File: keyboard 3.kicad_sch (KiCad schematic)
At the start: 9 parts, among them SW1 SW_Push, SW2 SW_Push, SW3 SW_Push, SW4 SW_Push, SW5 SW_Push, SW6 SW_Push, U1 XIAO-RP2040-DIP

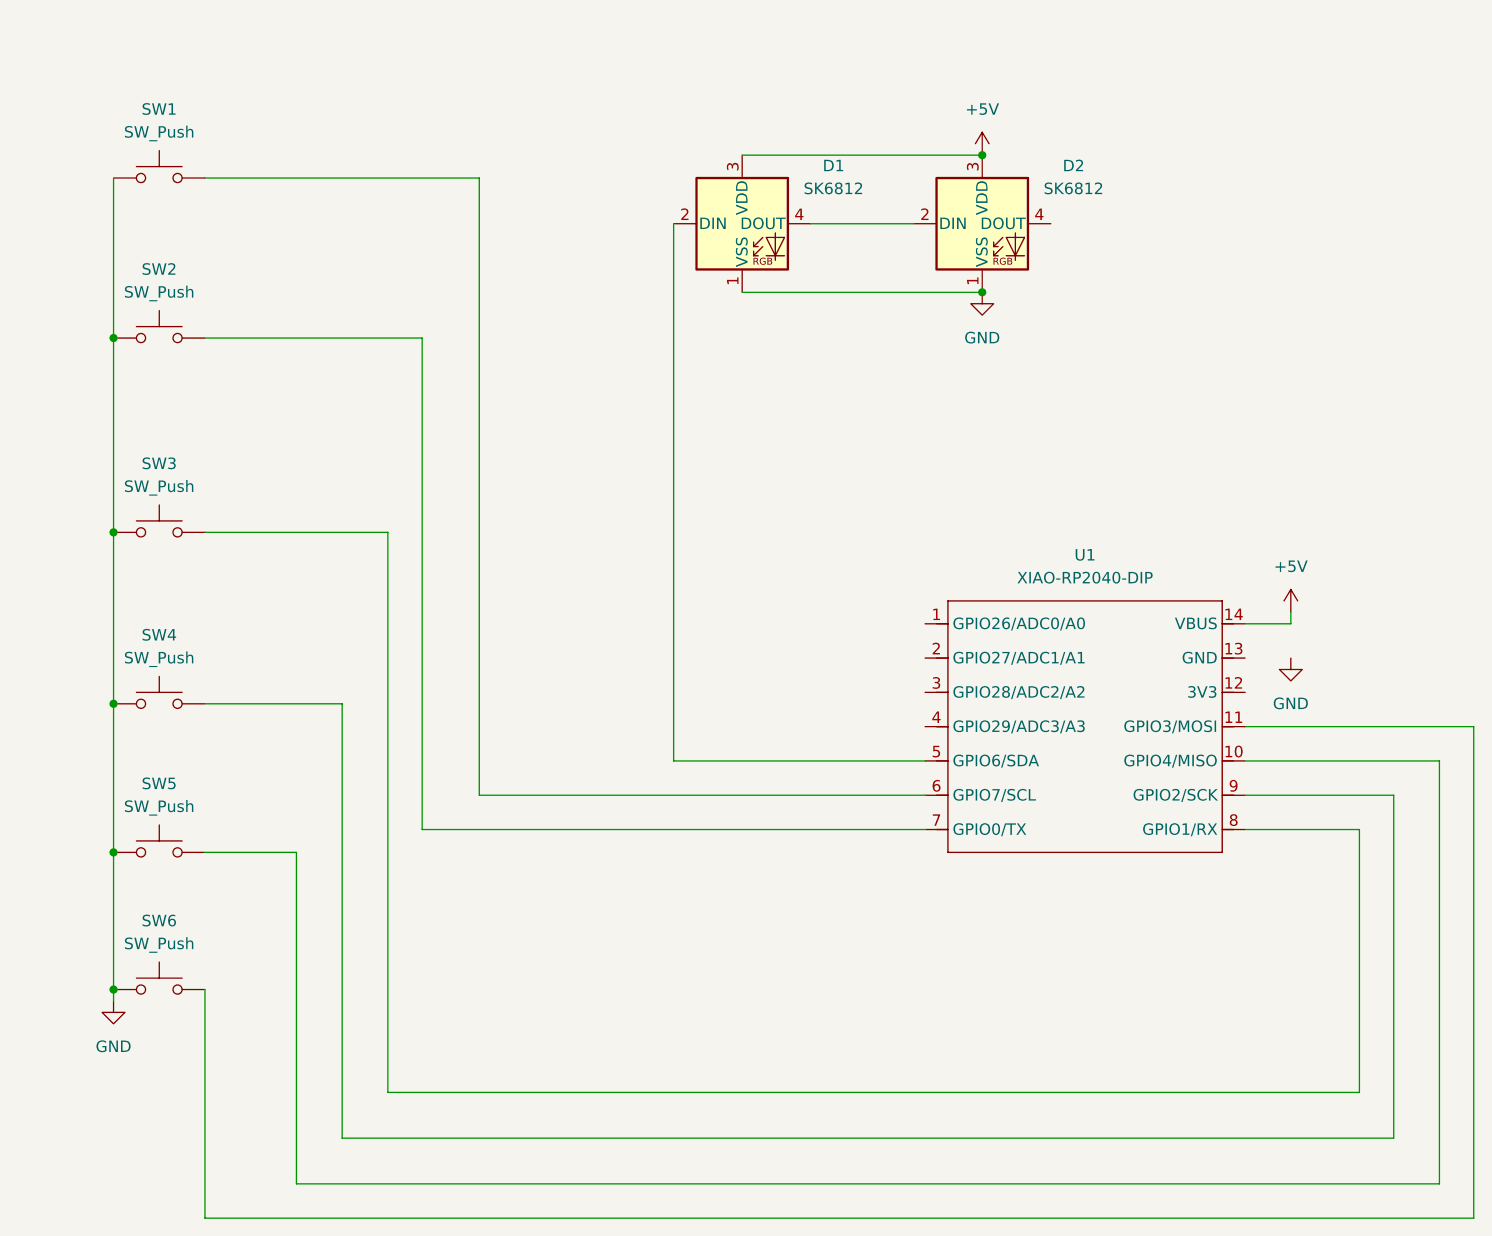
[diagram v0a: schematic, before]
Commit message: Add files via upload
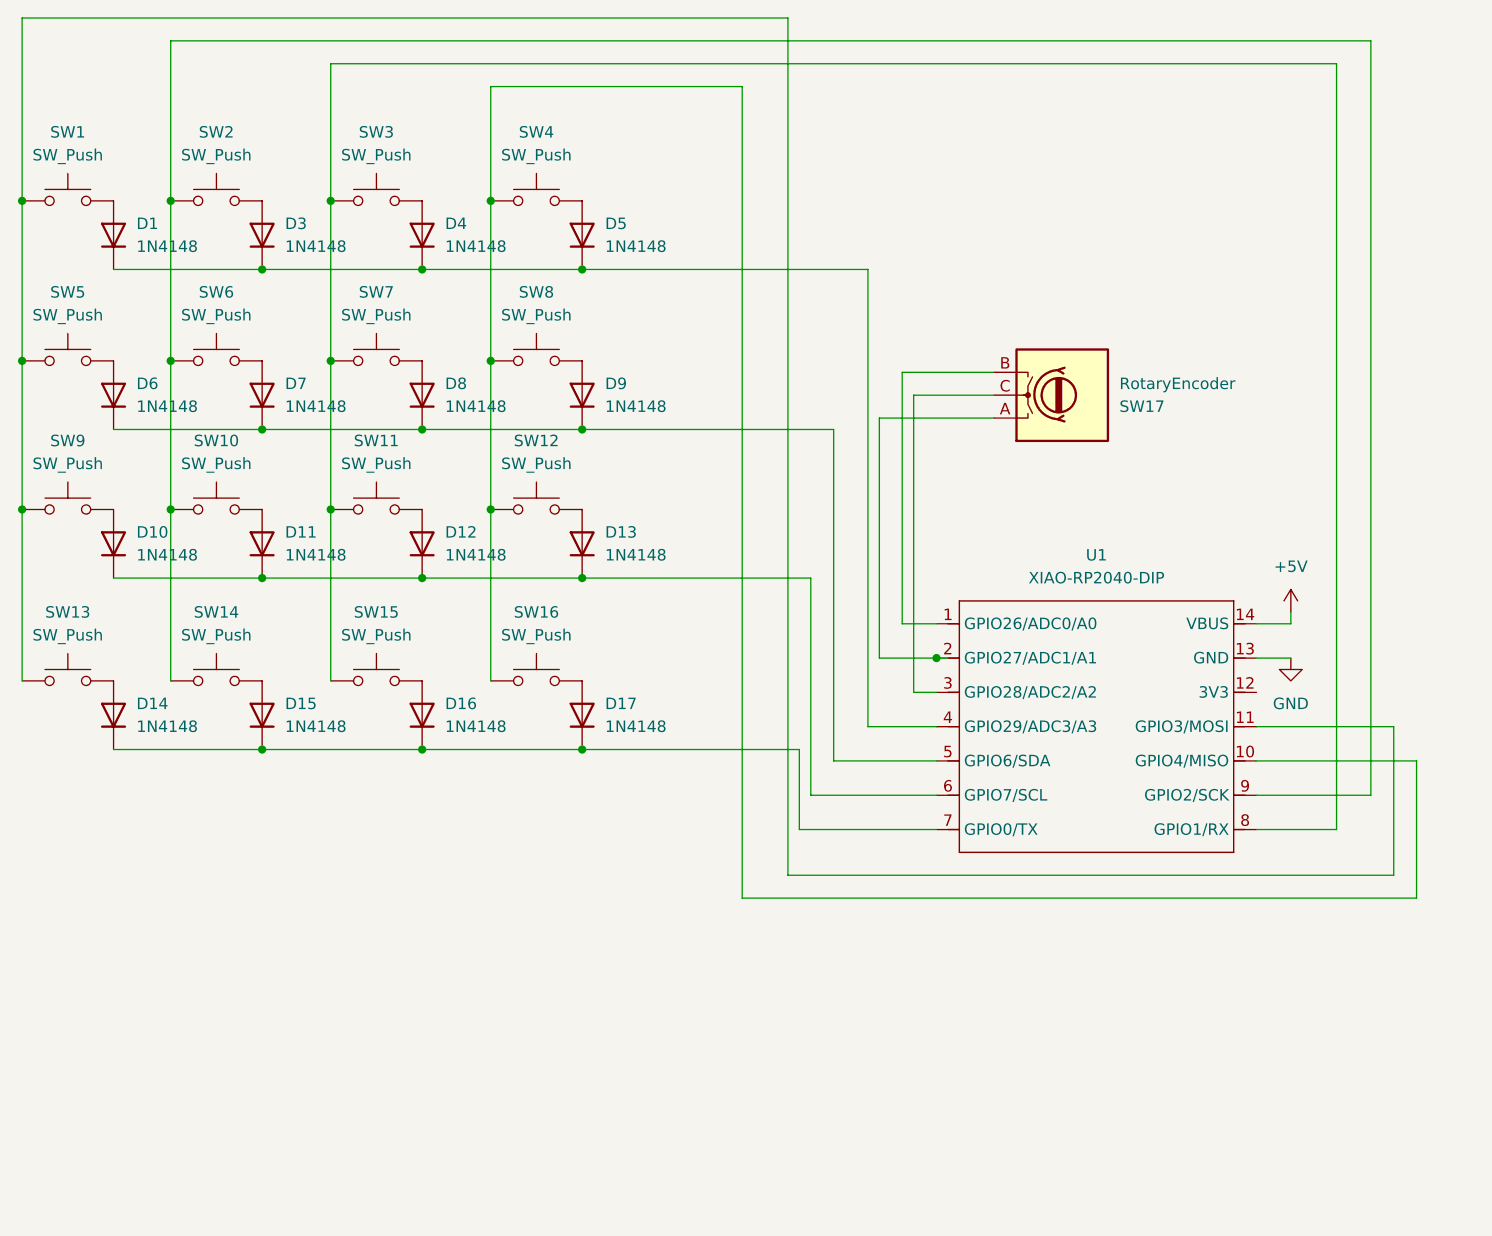
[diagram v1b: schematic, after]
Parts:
- removed D1, D2: SK6812, LED_SMD:LED_SK6812MINI_PLCC4_3.5x3.5mm_P1.75mm, symbol LED:SK6812
- added D1, D10, D11, D12, D13, D14, D15, D16, D17, D3, D4, D5, D6, D7, D8, D9: 1N4148, Diode_THT:D_DO-35_SOD27_P7.62mm_Horizontal, symbol Diode:1N4148
- added SW10, SW11, SW12, SW13, SW14, SW15, SW16, SW7, SW8, SW9: SW_Push, Button_Switch_Keyboard:SW_Cherry_MX_1.00u_PCB, symbol Switch:SW_Push
- added SW17: RotaryEncoder, Rotary_Encoder:RotaryEncoder_Alps_EC11E-Switch_Vertical_H20mm, symbol Device:RotaryEncoder
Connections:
- net GND: now also U1.13 (GND); no longer SW1.1, SW2.1, SW3.1, SW4.1, SW5.1, SW6.1
- net at U1.6 (GPIO7/SCL): now also D10.1 (K), D11.1 (K), D12.1 (K), D13.1 (K); no longer SW1.2
- net at U1.11 (GPIO3/MOSI): now also SW1.1, SW5.1, SW13.1, SW9.1; no longer SW6.2
- net at SW2.2: now also D3.2 (A); no longer U1.7 (GPIO0/TX)
- net at SW3.2: now also D4.2 (A); no longer U1.8 (GPIO1/RX)
- net at U1.9 (GPIO2/SCK): now also SW2.1, SW6.1, SW10.1, SW14.1; no longer SW4.2
- net at U1.10 (GPIO4/MISO): now also SW4.1, SW12.1, SW16.1, SW8.1; no longer SW5.2
- net at U1.5 (GPIO6/SDA): now also D6.1 (K), D7.1 (K), D8.1 (K), D9.1 (K)
- net at U1.1 (GPIO26/ADC0/A0): now also SW17.B
- net at U1.2 (GPIO27/ADC1/A1): now also SW17.A
- net at U1.3 (GPIO28/ADC2/A2): now also SW17.C
- net at U1.4 (GPIO29/ADC3/A3): now also D1.1 (K), D3.1 (K), D4.1 (K), D5.1 (K)
- new net: D13.2 (A), SW12.2
- new net: D6.2 (A), SW5.2
- new net: D11.2 (A), SW10.2
- new net: D1.2 (A), SW1.2
- new net: D17.2 (A), SW16.2
- new net: D8.2 (A), SW7.2
- new net: SW11.1, SW15.1, SW3.1, SW7.1, U1.8 (GPIO1/RX)
- new net: D12.2 (A), SW11.2
- new net: D9.2 (A), SW8.2
- new net: D7.2 (A), SW6.2
- new net: D5.2 (A), SW4.2
- new net: D16.2 (A), SW15.2
- new net: D14.1 (K), D15.1 (K), D16.1 (K), D17.1 (K), U1.7 (GPIO0/TX)
- new net: D10.2 (A), SW9.2
- new net: D15.2 (A), SW14.2
- new net: D14.2 (A), SW13.2
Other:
- moved on the sheet: U1
